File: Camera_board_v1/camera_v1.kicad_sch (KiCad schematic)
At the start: 27 parts, among them J1 Conn_01x01, J10 I2C1 Breakout, J7 FC Connector, J8 I2C1 Breakout, J9 I2C1 Breakout, U2 TLV74315, U3 TLV74328, X1 CAMERA_OV2640

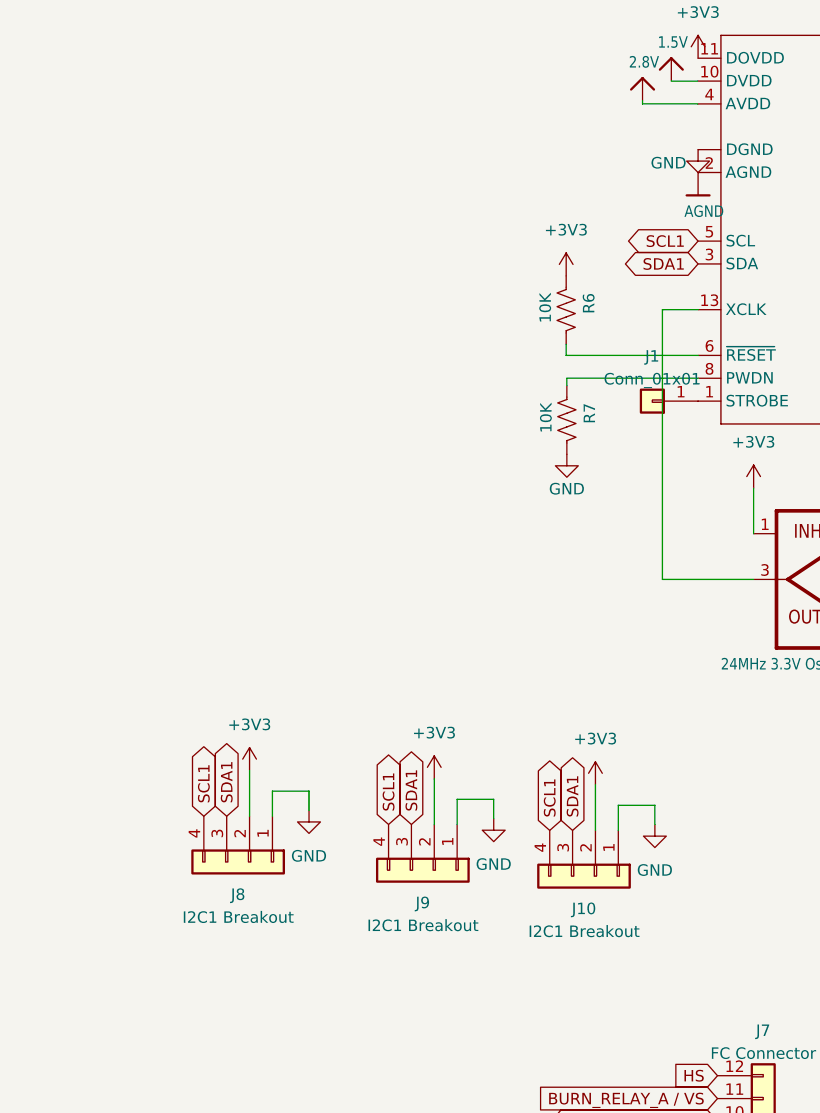
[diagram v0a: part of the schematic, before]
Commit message: Big Update of In Dev Boards
Mid Term update for all the boards being developed for use by the Irvington Team on Pleiades - Orpheus
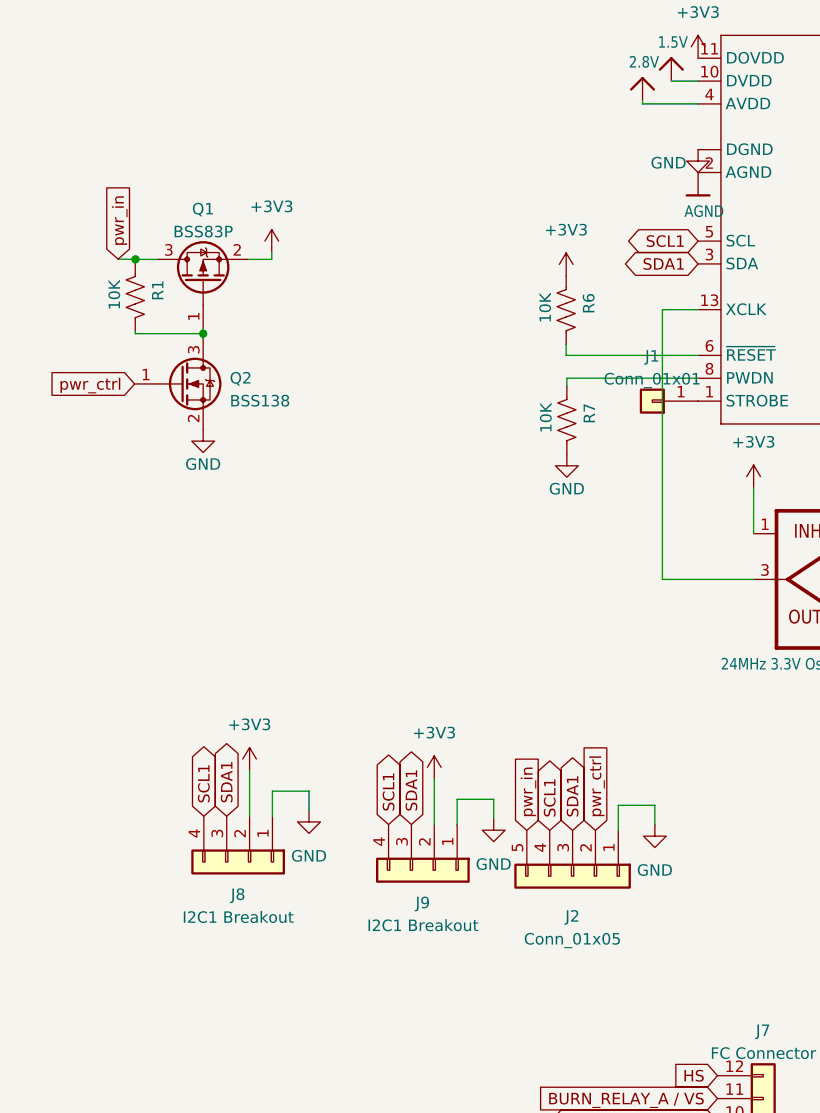
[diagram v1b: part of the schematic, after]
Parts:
- removed J10: I2C1 Breakout, Connector_PinHeader_2.54mm:PinHeader_1x04_P2.54mm_Vertical, symbol Connector_Generic:Conn_01x04
- added J2: Conn_01x05, Connector_PinHeader_2.54mm:PinHeader_1x05_P2.54mm_Vertical, symbol Connector_Generic:Conn_01x05
- added Q1: BSS83P, Package_TO_SOT_SMD:SOT-23, symbol Transistor_FET:BSS83P
- added Q2: BSS138, Package_TO_SOT_SMD:SOT-23, symbol Transistor_FET:BSS138
- added R1: 10K, Resistor_SMD:R_0603_1608Metric, symbol Device:R_US
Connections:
- net +3V3: now also Q1.2 (S)
- net GND: now also J2.1 (Pin_1), Q2.2 (S)
- net SCL1: now also J2.4 (Pin_4)
- net SDA1: now also J2.3 (Pin_3)
- new net: Q1.1 (G), Q2.3 (D), R1.2
- new net pwr_ctrl: J2.2 (Pin_2), Q2.1 (G)
- new net pwr_in: J2.5 (Pin_5), Q1.3 (D), R1.1
